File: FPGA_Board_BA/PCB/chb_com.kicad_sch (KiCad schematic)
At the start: 4 parts, among them J1401 Plug_Terminal_2x12pin, J1402 Plug_Terminal_2x12pin, J1403 Plug_Terminal_2x12pin, J1404 Plug_Terminal_2x12pin

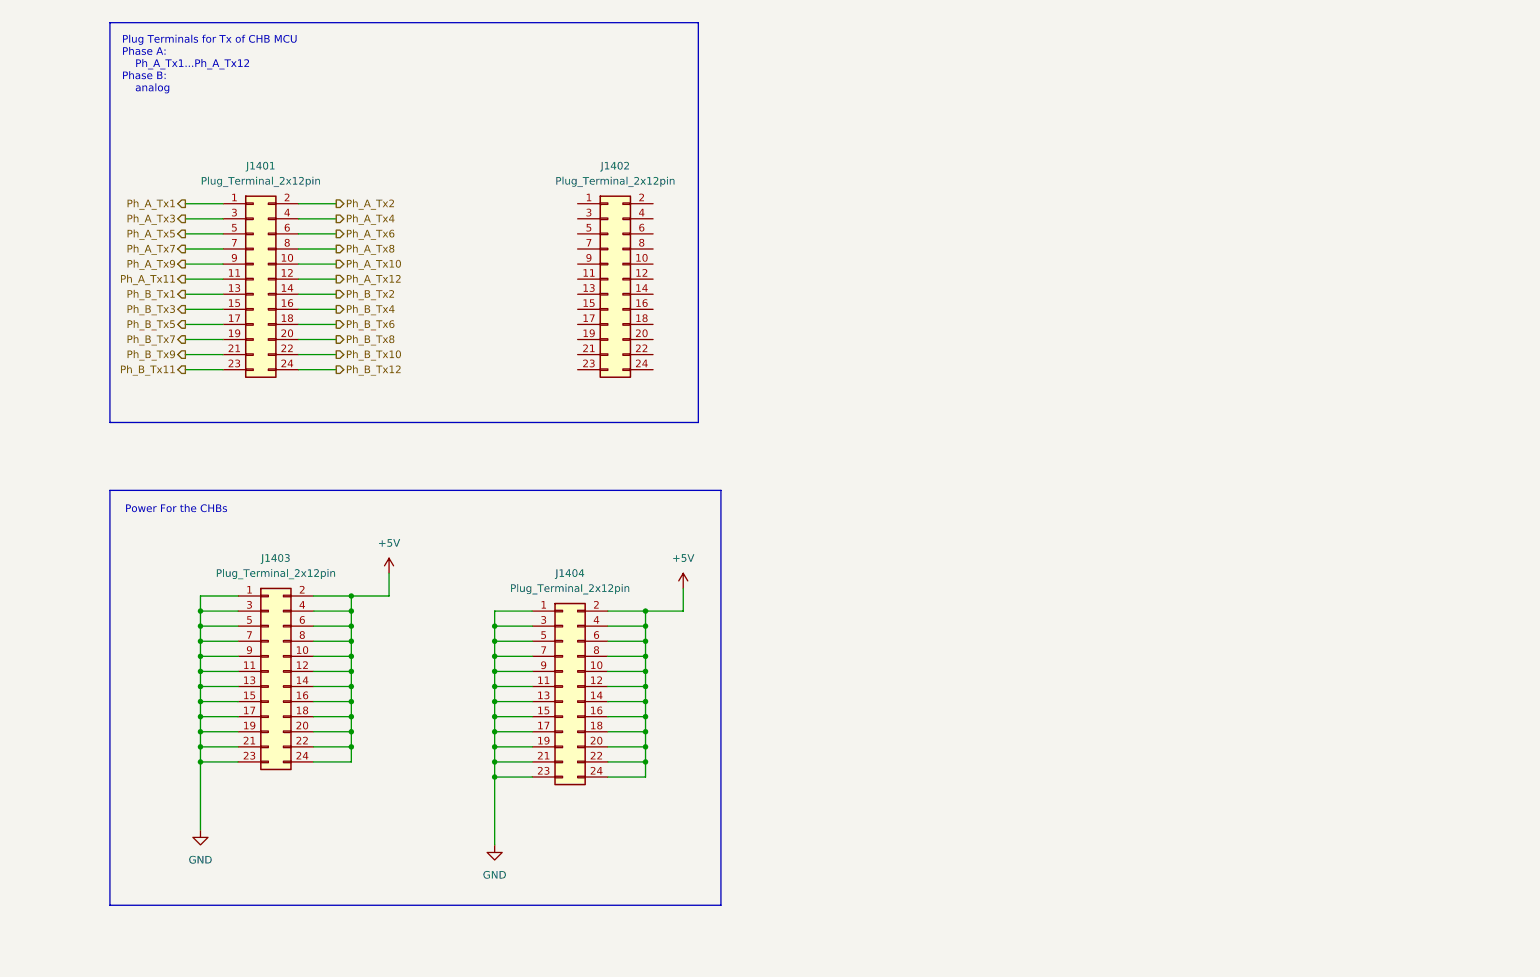
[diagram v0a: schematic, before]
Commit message: schematic almost ready
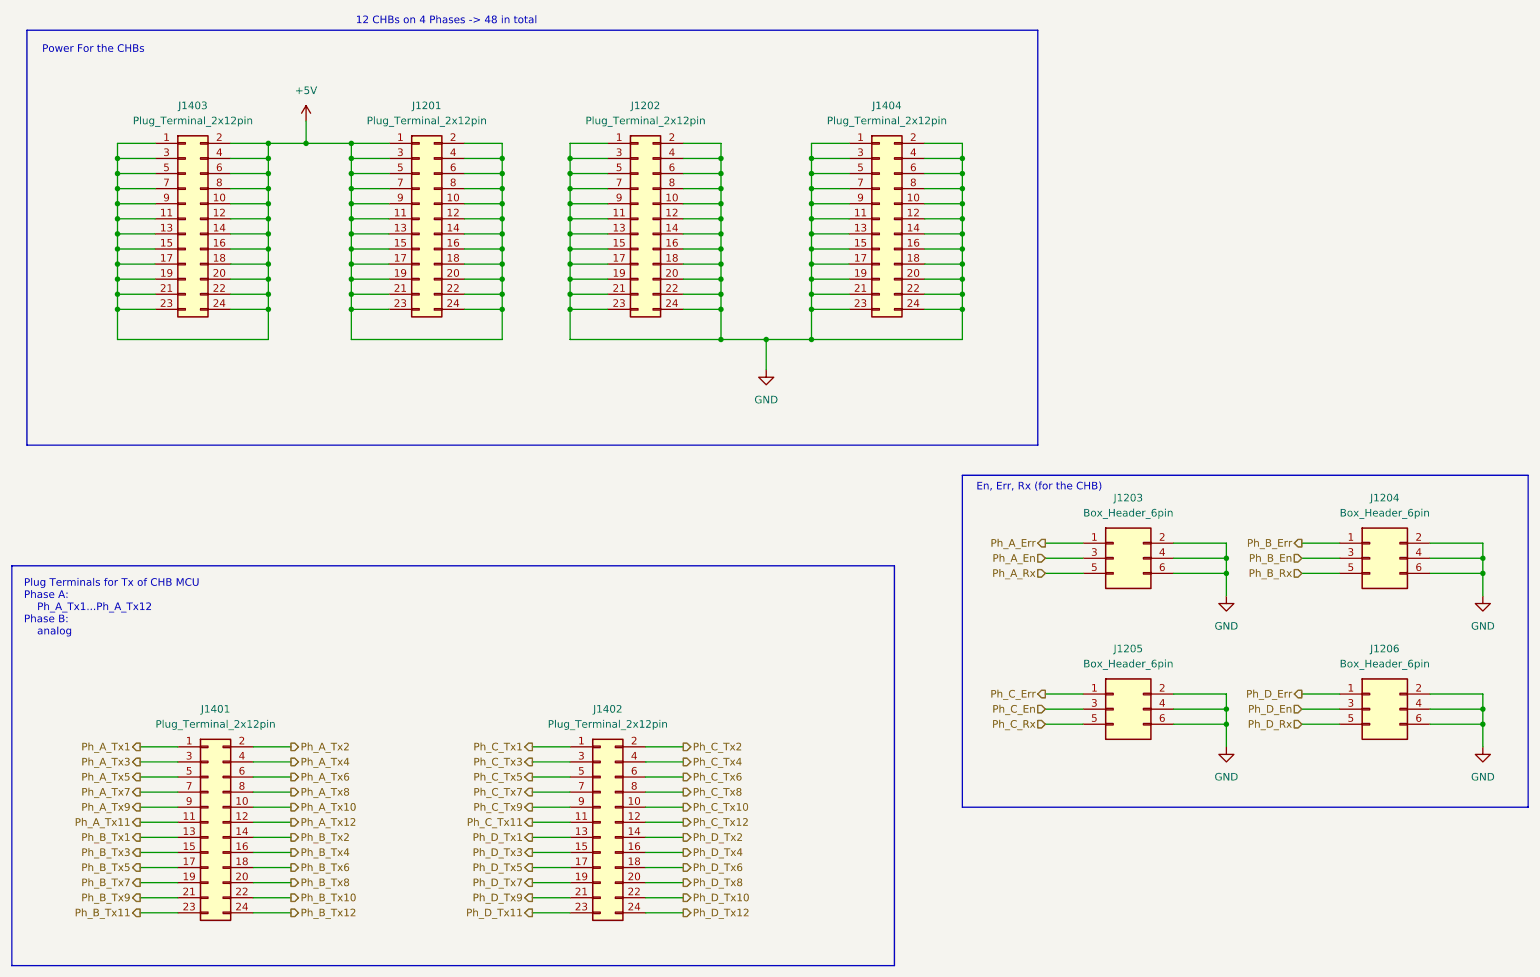
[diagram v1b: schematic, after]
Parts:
- added J1201, J1202: Plug_Terminal_2x12pin, MYLIB_Misc:DMCV 1,5_12-G1F-3,5-LR P20THR, symbol MYLIB_Misc:Plug_Terminal_2x12pin
- added J1203, J1204, J1205, J1206: Box_Header_6pin, Connector_IDC:IDC-Header_2x03_P2.54mm_Vertical, symbol MYLIB_Misc:Box_Header_6pin
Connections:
- net +5V: now also J1403.1, J1403.11, J1403.13, J1403.15, J1403.17, J1403.19, J1403.21, J1403.23, J1403.3, J1403.5, J1403.7, J1403.9, J1201.1, J1201.10, J1201.11, J1201.12, J1201.13, J1201.14, J1201.15, J1201.16, J1201.17, J1201.18, J1201.19, J1201.2, J1201.20, J1201.21, J1201.22, J1201.23, J1201.24, J1201.3, J1201.4, J1201.5, J1201.6, J1201.7, J1201.8, J1201.9; no longer J1404.10, J1404.12, J1404.14, J1404.16, J1404.18, J1404.2, J1404.20, J1404.22, J1404.24, J1404.4, J1404.6, J1404.8
- net GND: now also J1404.10, J1404.12, J1404.14, J1404.16, J1404.18, J1404.2, J1404.20, J1404.22, J1404.24, J1404.4, J1404.6, J1404.8, J1202.1, J1202.10, J1202.11, J1202.12, J1202.13, J1202.14, J1202.15, J1202.16, J1202.17, J1202.18, J1202.19, J1202.2, J1202.20, J1202.21, J1202.22, J1202.23, J1202.24, J1202.3, J1202.4, J1202.5, J1202.6, J1202.7, J1202.8, J1202.9, J1203.2 (Pin_2), J1203.4 (Pin_4), J1203.6 (Pin_6), J1204.2 (Pin_2), J1204.4 (Pin_4), J1204.6 (Pin_6), J1205.2 (Pin_2), J1205.4 (Pin_4), J1205.6 (Pin_6), J1206.2 (Pin_2), J1206.4 (Pin_4), J1206.6 (Pin_6); no longer J1403.1, J1403.11, J1403.13, J1403.15, J1403.17, J1403.19, J1403.21, J1403.23, J1403.3, J1403.5, J1403.7, J1403.9
- net Ph_C_Tx1: now reaches J1402.1
- net Ph_C_Tx10: now reaches J1402.10
- net Ph_C_Tx11: now reaches J1402.11
- net Ph_C_Tx12: now reaches J1402.12
- net Ph_D_Tx1: now reaches J1402.13
- net Ph_D_Tx2: now reaches J1402.14
- net Ph_D_Tx3: now reaches J1402.15
- net Ph_D_Tx4: now reaches J1402.16
- net Ph_D_Tx5: now reaches J1402.17
- net Ph_D_Tx6: now reaches J1402.18
- net Ph_D_Tx7: now reaches J1402.19
- net Ph_C_Tx2: now reaches J1402.2
- net Ph_D_Tx8: now reaches J1402.20
- net Ph_D_Tx9: now reaches J1402.21
- net Ph_D_Tx10: now reaches J1402.22
- net Ph_D_Tx11: now reaches J1402.23
- net Ph_D_Tx12: now reaches J1402.24
- net Ph_C_Tx3: now reaches J1402.3
- net Ph_C_Tx4: now reaches J1402.4
- net Ph_C_Tx5: now reaches J1402.5
- net Ph_C_Tx6: now reaches J1402.6
- net Ph_C_Tx7: now reaches J1402.7
- net Ph_C_Tx8: now reaches J1402.8
- net Ph_C_Tx9: now reaches J1402.9
- new net Ph_A_En: J1203.3 (Pin_3)
- new net Ph_A_Err: J1203.1 (Pin_1)
- new net Ph_A_Rx: J1203.5 (Pin_5)
- new net Ph_B_En: J1204.3 (Pin_3)
- new net Ph_B_Err: J1204.1 (Pin_1)
- new net Ph_B_Rx: J1204.5 (Pin_5)
- new net Ph_C_En: J1205.3 (Pin_3)
- new net Ph_C_Err: J1205.1 (Pin_1)
- new net Ph_C_Rx: J1205.5 (Pin_5)
- new net Ph_D_En: J1206.3 (Pin_3)
- new net Ph_D_Err: J1206.1 (Pin_1)
- new net Ph_D_Rx: J1206.5 (Pin_5)
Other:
- note added: "12 CHBs on 4 Phases -> 48 in total"
- note added: "En, Err, Rx (for the CHB)"
- moved on the sheet: J1401, J1402, J1403, J1404
